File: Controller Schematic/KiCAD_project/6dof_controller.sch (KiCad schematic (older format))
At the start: 111 parts, among them J1 Screw_Terminal_01x03, J10 Conn_02x13_Top_Bottom, J2 DS-201, J3 RJ45, J4 Conn_02x13_Top_Bottom, J5 Conn_02x13_Top_Bottom, J6 Conn_02x13_Top_Bottom, J7 Conn_02x05_Top_Bottom, J8 Conn_02x13_Top_Bottom, J9 Conn_02x13_Top_Bottom, U1 ESP32_DevKit_V1_DOIT, U10 4N35, U11 4N35, U12 4N35, U13 4N35, U14 4N35, U15 4N35, U2 4N35, U3 MCP23SigIn1M17_SP, U4 4N35, U5 4N35, U6 4N35, U7 4N35, U8 4N35, U9 4N35

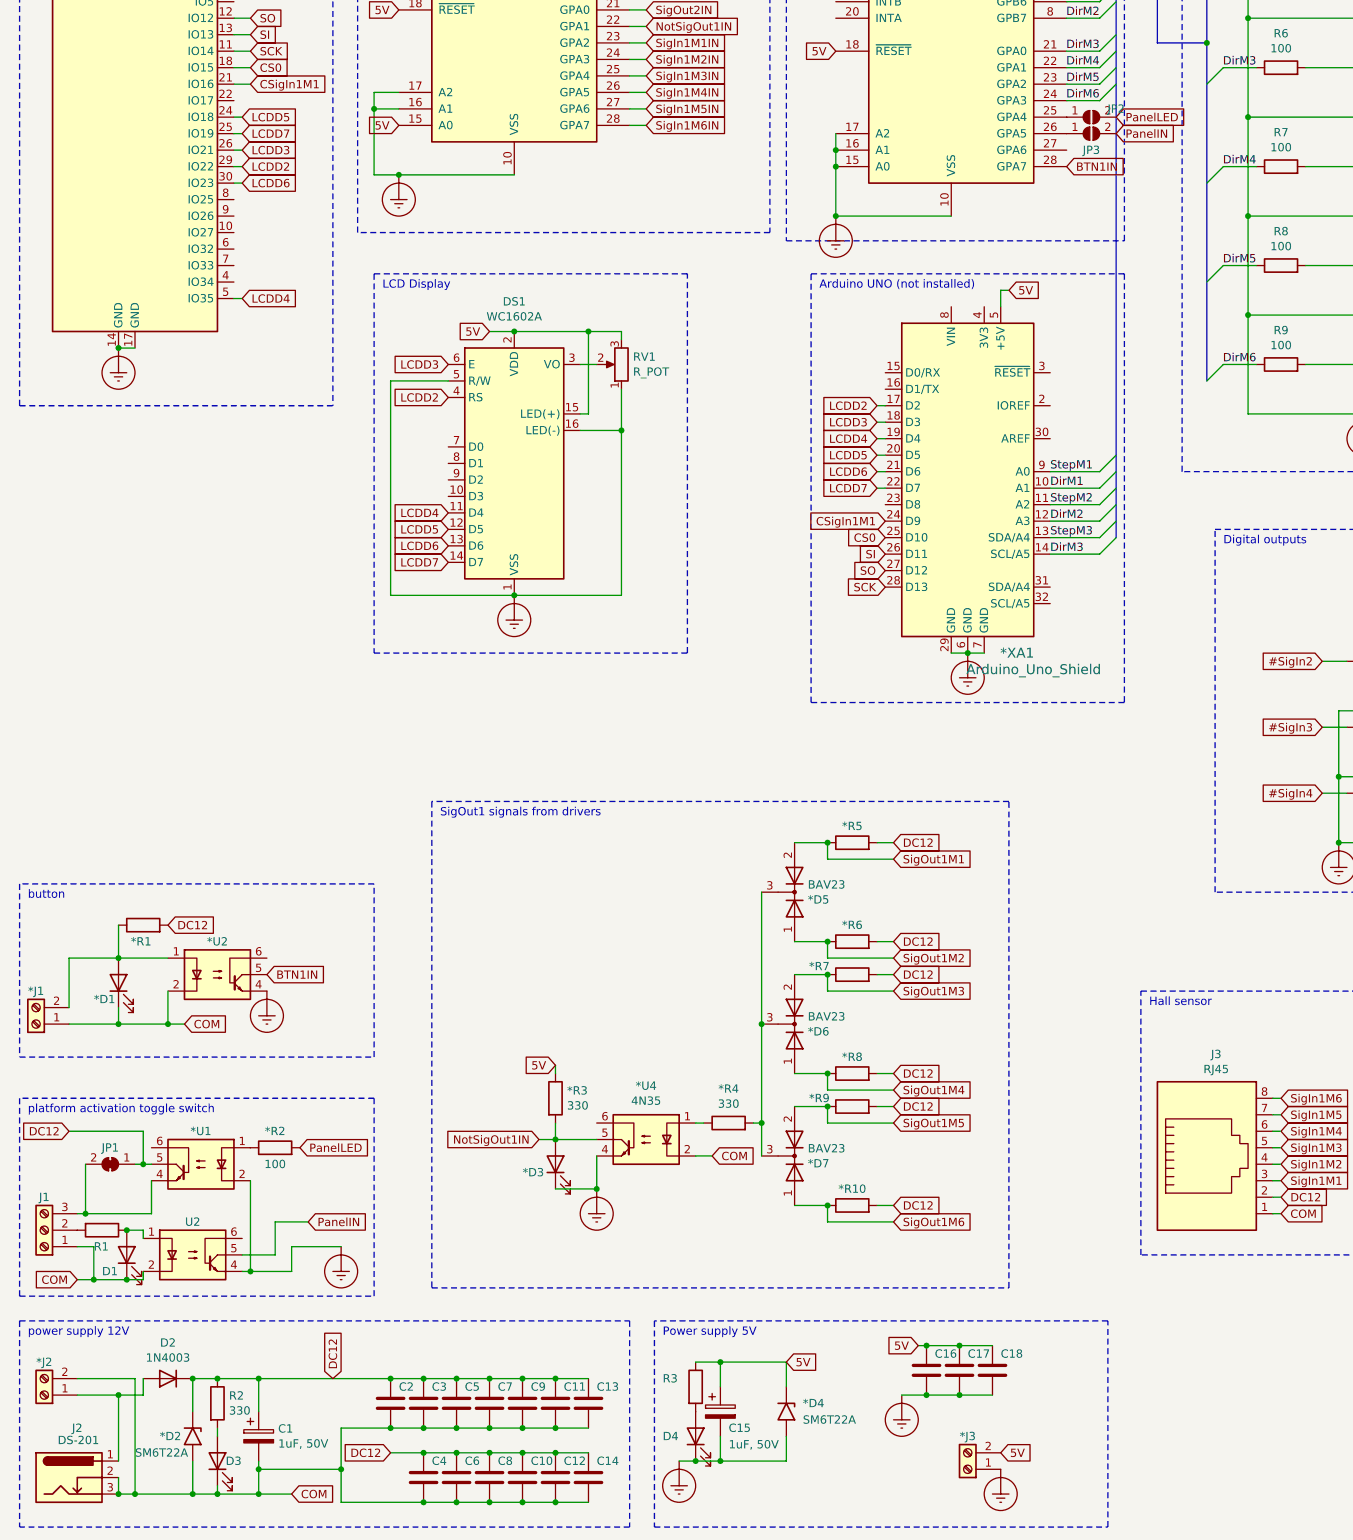
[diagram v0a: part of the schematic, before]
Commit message: project updated
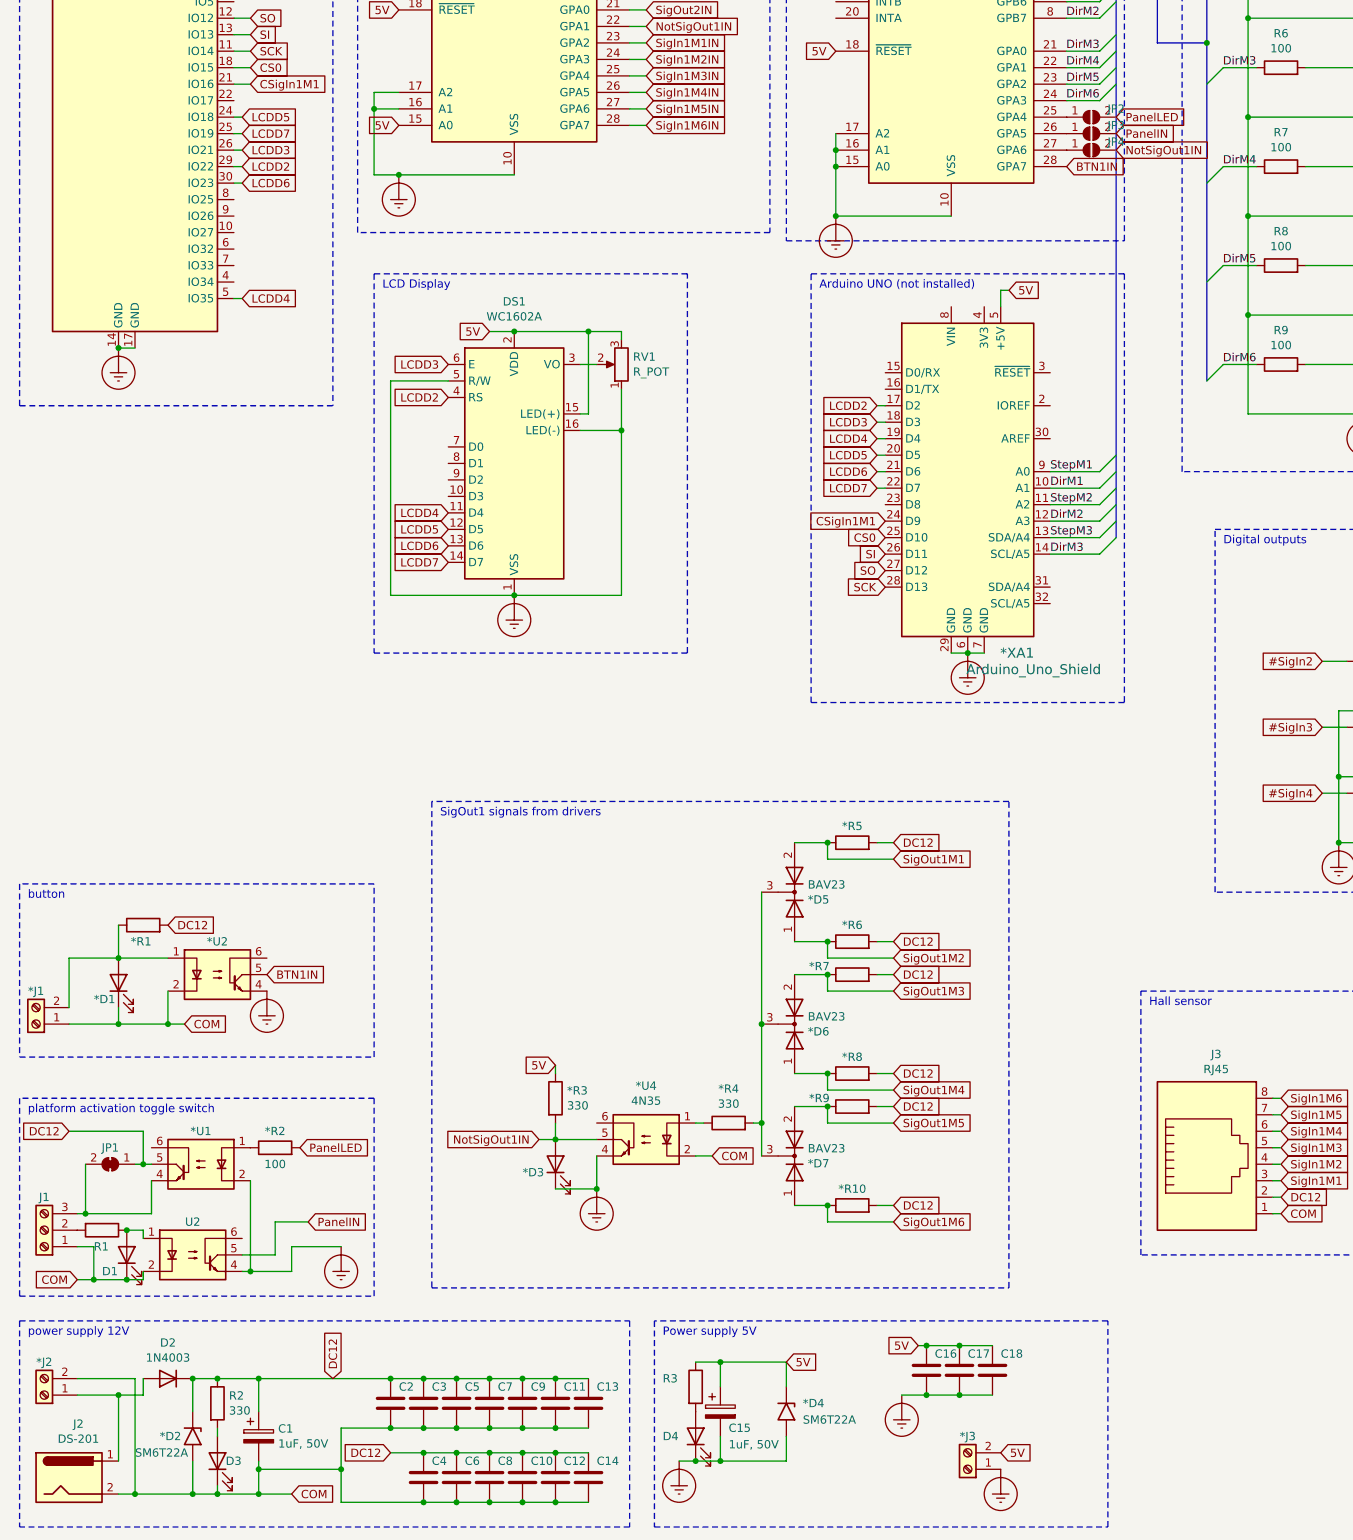
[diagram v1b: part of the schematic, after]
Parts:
- removed J2: DS-201, Connector_BarrelJack:BarrelJack_CUI_PJ-063AH_Horizontal, symbol Connector:Barrel_Jack_Switch_Pin3Ring
- added J2: DS-201, Connector_BarrelJack:BarrelJack_CUI_PJ-063AH_Horizontal, symbol Connector:Barrel_Jack
- added JP4: SolderJumper_2_Open, Jumper:SolderJumper-2_P1.3mm_Open_Pad1.0x1.5mm, symbol Jumper:SolderJumper_2_Open
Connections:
- net COM: now also J2.2
- net NotSigOut1IN: now also JP4.2 (B)
- net at U3.27 (GPA6): now also JP4.1 (A)
- net at *J2.1 (Pin_1), D2.2 (A): now also J2.1
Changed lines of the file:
@@
 Wire Wire Line
 	1200 10650 1200 10250
-$Comp
-L Connector:Barrel_Jack_Switch_Pin3Ring J2
-U 1 1 601FD643
-P 900 10750
-F 0 "J2" H 950 11050 50  0000 C CNN
-F 1 "DS-201" H 957 10976 50  0000 C CNN
-F 2 "Connector_BarrelJack:BarrelJack_CUI_PJ-063AH_Horizontal" H 950 10710 50  0001 C CNN
-F 3 "https://www.chipdip.ru/product/ds-201" H 950 10710 50  0001 C CNN
-	1    900  10750
-	1    0    0    -1
-$EndComp
 Text GLabel 2500 10150 1    50   Input ~ 0
 DC12
@@
 Wire Wire Line
 	11200 4100 11300 4100
-Wire Wire Line
-	1200 10750 1200 10850
-Connection ~ 1200 10850
 Wire Bus Line
 	7500 650  7500 2050
@@
 	2550 10900 3050 10900
 Connection ~ 2550 10700
-$Comp
-L Jumper:SolderJumper_2_Open JP2
-U 1 1 602EB81E
-P 7100 2500
-F 0 "JP2" H 7250 2550 50  0000 C CNN
-F 1 "SolderJumper_2_Open" H 7100 2614 50  0001 C CNN
-F 2 "Jumper:SolderJumper-2_P1.3mm_Open_Pad1.0x1.5mm" H 7100 2500 50  0001 C CNN
-F 3 "~" H 7100 2500 50  0001 C CNN
-	1    7100 2500
-	1    0    0    -1
-$EndComp
-$Comp
-L Jumper:SolderJumper_2_Open JP3
-U 1 1 602ED0FE
-P 7100 2600
-F 0 "JP3" H 7100 2500 50  0000 C CNN
-F 1 "SolderJumper_2_Open" H 7100 2714 50  0001 C CNN
-F 2 "Jumper:SolderJumper-2_P1.3mm_Open_Pad1.0x1.5mm" H 7100 2600 50  0001 C CNN
-F 3 "~" H 7100 2600 50  0001 C CNN
-	1    7100 2600
-	1    0    0    -1
-$EndComp
 Text GLabel 7250 2500 2    50   Input ~ 0
 PanelLED
@@
 Wire Bus Line
 	7250 650  7250 5050
+$Comp
+L Jumper:SolderJumper_2_Open JP4
+U 1 1 5FCE05BC
+P 7100 2700
+F 0 "JP4" H 7250 2750 50  0000 C CNN
+F 1 "SolderJumper_2_Open" H 7100 2814 50  0001 C CNN
+F 2 "Jumper:SolderJumper-2_P1.3mm_Open_Pad1.0x1.5mm" H 7100 2700 50  0001 C CNN
+F 3 "~" H 7100 2700 50  0001 C CNN
+	1    7100 2700
+	1    0    0    -1
+$EndComp
+Text GLabel 7250 2700 2    50   Input ~ 0
+NotSigOut1IN
+$Comp
+L Jumper:SolderJumper_2_Open JP3
+U 1 1 602ED0FE
+P 7100 2600
+F 0 "JP3" H 7250 2650 50  0000 C CNN
+F 1 "SolderJumper_2_Open" H 7100 2714 50  0001 C CNN
+F 2 "Jumper:SolderJumper-2_P1.3mm_Open_Pad1.0x1.5mm" H 7100 2600 50  0001 C CNN
+F 3 "~" H 7100 2600 50  0001 C CNN
+	1    7100 2600
+	1    0    0    -1
+$EndComp
+$Comp
+L Jumper:SolderJumper_2_Open JP2
+U 1 1 602EB81E
+P 7100 2500
+F 0 "JP2" H 7250 2550 50  0000 C CNN
+F 1 "SolderJumper_2_Open" H 7100 2614 50  0001 C CNN
+F 2 "Jumper:SolderJumper-2_P1.3mm_Open_Pad1.0x1.5mm" H 7100 2500 50  0001 C CNN
+F 3 "~" H 7100 2500 50  0001 C CNN
+	1    7100 2500
+	1    0    0    -1
+$EndComp
+$Comp
+L Connector:Barrel_Jack J2
+U 1 1 5FCE9EE6
+P 900 10750
+F 0 "J2" H 957 11075 50  0000 C CNN
+F 1 "DS-201" H 957 10984 50  0000 C CNN
+F 2 "Connector_BarrelJack:BarrelJack_CUI_PJ-063AH_Horizontal" H 950 10710 50  0001 C CNN
+F 3 "https://www.chipdip.ru/product/ds-201" H 950 10710 50  0001 C CNN
+	1    900  10750
+	1    0    0    -1
+$EndComp
 $EndSCHEMATC
